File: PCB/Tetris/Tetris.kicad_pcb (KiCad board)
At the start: 2 copper layers, 101.6 x 53.3 mm, 27 parts, among them J1 Power, J2 PWM, J3 Analog, J4 PWM, J5 Analog, J6 Communication, J7 Digital, M1 RGBMatrix, M2 RGBMatrix, SW1 SW_Push, SW2 SW_Push, SW3 SW_Push, SW4 SW_Push, SW5 SW_Push, SW6 SW_Push, SW7 SW_Push

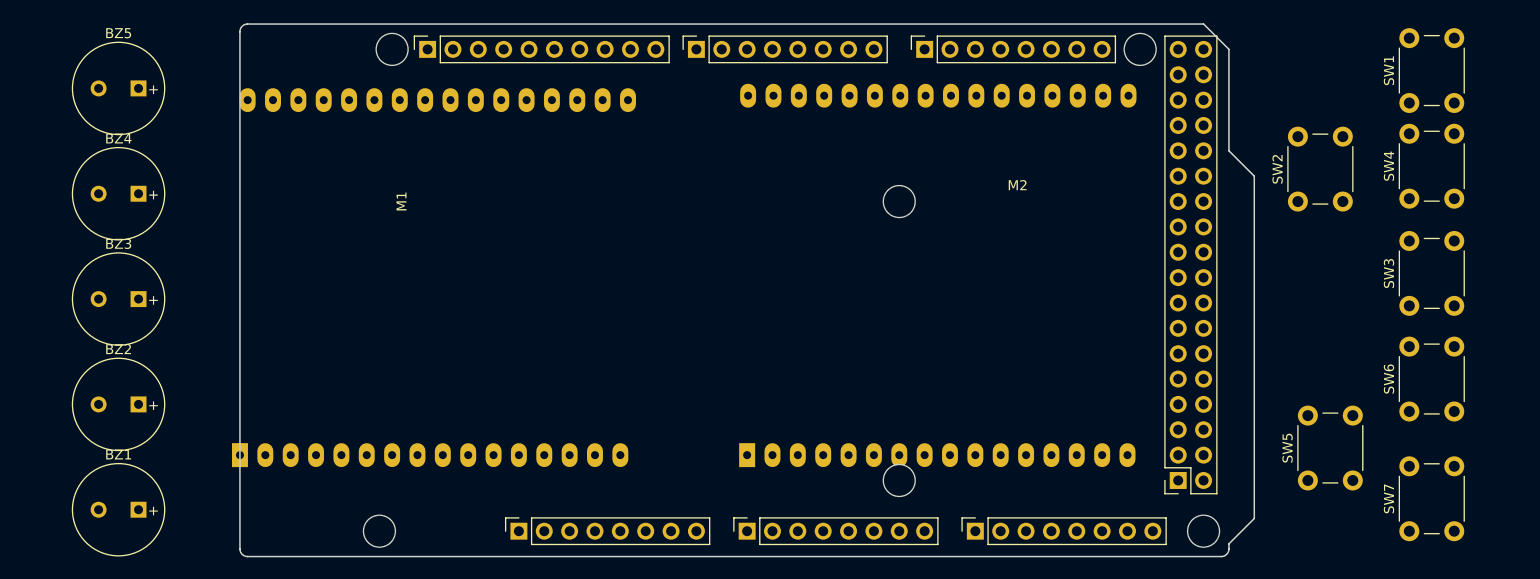
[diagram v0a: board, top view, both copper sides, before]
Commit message: sync
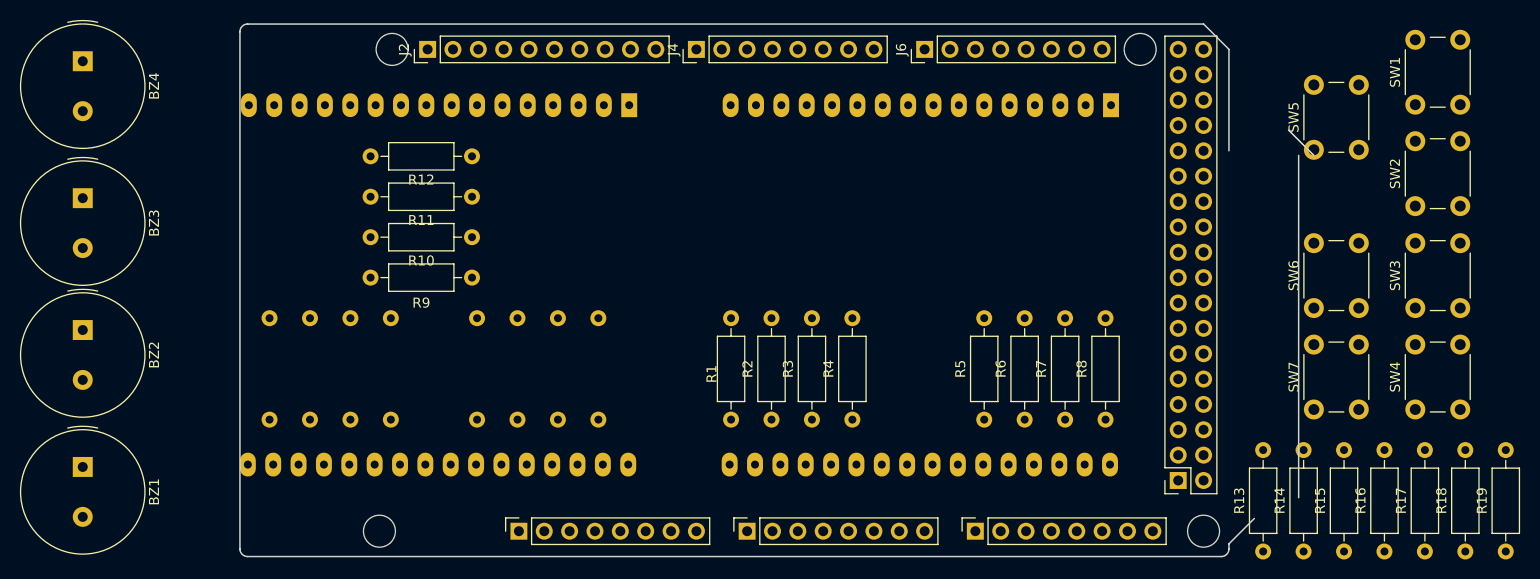
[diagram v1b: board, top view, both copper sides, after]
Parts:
- removed BZ5: Active Buzzer, Buzzer_Beeper:MagneticBuzzer_PUI_AT-0927-TT-6-R
- removed MH3, MH4: MountingHole_3.2mm, Arduino_MountingHole:MountingHole_3.2mm
- added R1: 110, Resistor_THT:R_Axial_DIN0207_L6.3mm_D2.5mm_P10.16mm_Horizontal, F.Cu at (149.2, 86.3)
- added R10: 220, Resistor_THT:R_Axial_DIN0207_L6.3mm_D2.5mm_P10.16mm_Horizontal, F.Cu at (123.2, 68.0)
- added R11: 220, Resistor_THT:R_Axial_DIN0207_L6.3mm_D2.5mm_P10.16mm_Horizontal, F.Cu at (123.2, 64.0)
- added R12: 220, Resistor_THT:R_Axial_DIN0207_L6.3mm_D2.5mm_P10.16mm_Horizontal, F.Cu at (123.2, 59.9)
- added R13: 10k, Resistor_THT:R_Axial_DIN0207_L6.3mm_D2.5mm_P10.16mm_Horizontal, F.Cu at (202.5, 99.5)
- added R14: 10k, Resistor_THT:R_Axial_DIN0207_L6.3mm_D2.5mm_P10.16mm_Horizontal, F.Cu at (206.5, 99.5)
- added R15: 10k, Resistor_THT:R_Axial_DIN0207_L6.3mm_D2.5mm_P10.16mm_Horizontal, F.Cu at (210.6, 99.5)
- added R16: 10k, Resistor_THT:R_Axial_DIN0207_L6.3mm_D2.5mm_P10.16mm_Horizontal, F.Cu at (214.6, 99.5)
- added R17: 10k, Resistor_THT:R_Axial_DIN0207_L6.3mm_D2.5mm_P10.16mm_Horizontal, F.Cu at (218.7, 99.5)
- added R18: 10k, Resistor_THT:R_Axial_DIN0207_L6.3mm_D2.5mm_P10.16mm_Horizontal, F.Cu at (222.7, 99.5)
- added R19: 10k, Resistor_THT:R_Axial_DIN0207_L6.3mm_D2.5mm_P10.16mm_Horizontal, F.Cu at (226.8, 99.5)
- added R2: 110, Resistor_THT:R_Axial_DIN0207_L6.3mm_D2.5mm_P10.16mm_Horizontal, F.Cu at (153.2, 86.3)
- added R20: 110, Resistor_THT:R_Axial_DIN0207_L6.3mm_D2.5mm_P10.16mm_Horizontal, B.Cu at (135.9, 86.3)
- added R21: 110, Resistor_THT:R_Axial_DIN0207_L6.3mm_D2.5mm_P10.16mm_Horizontal, B.Cu at (131.8, 86.3)
- added R22: 110, Resistor_THT:R_Axial_DIN0207_L6.3mm_D2.5mm_P10.16mm_Horizontal, B.Cu at (127.8, 86.3)
- added R23: 110, Resistor_THT:R_Axial_DIN0207_L6.3mm_D2.5mm_P10.16mm_Horizontal, B.Cu at (123.7, 86.3)
- added R24: 110, Resistor_THT:R_Axial_DIN0207_L6.3mm_D2.5mm_P10.16mm_Horizontal, B.Cu at (115.1, 86.3)
- added R25: 110, Resistor_THT:R_Axial_DIN0207_L6.3mm_D2.5mm_P10.16mm_Horizontal, B.Cu at (111.1, 86.3)
- added R26: 110, Resistor_THT:R_Axial_DIN0207_L6.3mm_D2.5mm_P10.16mm_Horizontal, B.Cu at (107.0, 86.3)
- added R27: 110, Resistor_THT:R_Axial_DIN0207_L6.3mm_D2.5mm_P10.16mm_Horizontal, B.Cu at (103.0, 86.3)
- added R3: 110, Resistor_THT:R_Axial_DIN0207_L6.3mm_D2.5mm_P10.16mm_Horizontal, F.Cu at (157.3, 86.3)
- added R4: 110, Resistor_THT:R_Axial_DIN0207_L6.3mm_D2.5mm_P10.16mm_Horizontal, F.Cu at (161.3, 86.3)
- added R5: 110, Resistor_THT:R_Axial_DIN0207_L6.3mm_D2.5mm_P10.16mm_Horizontal, F.Cu at (174.5, 86.3)
- added R6: 110, Resistor_THT:R_Axial_DIN0207_L6.3mm_D2.5mm_P10.16mm_Horizontal, F.Cu at (178.6, 86.3)
- added R7: 110, Resistor_THT:R_Axial_DIN0207_L6.3mm_D2.5mm_P10.16mm_Horizontal, F.Cu at (182.6, 86.3)
- added R8: 110, Resistor_THT:R_Axial_DIN0207_L6.3mm_D2.5mm_P10.16mm_Horizontal, F.Cu at (186.7, 86.3)
- added R9: 220, Resistor_THT:R_Axial_DIN0207_L6.3mm_D2.5mm_P10.16mm_Horizontal, F.Cu at (123.2, 72.1)
- BZ1, BZ2, BZ3, BZ4: footprint Buzzer_Beeper:MagneticBuzzer_PUI_AT-0927-TT-6-R -> Buzzer_Beeper:Buzzer_TDK_PS1240P02BT_D12.2mm_H6.5mm
- J2: footprint Connector_PinSocket_2.54mm:PinSocket_1x10_P2.54mm_Vertical -> Connector_PinHeader_2.54mm:PinHeader_1x10_P2.54mm_Vertical
- J4, J6: footprint Connector_PinSocket_2.54mm:PinSocket_1x08_P2.54mm_Vertical -> Connector_PinHeader_2.54mm:PinHeader_1x08_P2.54mm_Vertical
- moved M2 50.0 mm to (119.9, 72.8), turned to 180 degrees
- moved M1 49.6 mm to (168.1, 72.8), turned to 180 degrees
- moved SW5 33.1 mm to (207.6, 59.3)
- moved SW4 21.1 mm to (217.7, 85.3)
- moved SW7 15.5 mm to (207.6, 85.3)
- moved BZ4 14.4 mm to (84.3, 50.4), turned to -90 degrees
- moved SW6 14.1 mm to (207.6, 75.1)
- moved SW2 11.8 mm to (217.7, 64.9)
- moved BZ3 11.6 mm to (84.3, 64.1), turned to -90 degrees
- moved BZ2 9.31 mm to (84.3, 77.3), turned to -90 degrees
- moved BZ1 7.04 mm to (84.3, 91.0), turned to -90 degrees
- moved SW3 0.64 mm to (217.7, 75.1)
- moved SW1 0.62 mm to (217.7, 54.7)
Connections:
- M1 pad 10: /1 -> /10
- M1 pad 11: /1 -> /11
- M1 pad 12: /1 -> /12
- M1 pad 13: /1 -> /13
- M1 pad 14: /1 -> /14
- M1 pad 15: /1 -> /15
- M1 pad 16: /1 -> /16
- M1 pad 2: /1 -> /2
- M1 pad 21: /1 -> /21
- M1 pad 22: /1 -> /22
- M1 pad 23: /1 -> /23
- M1 pad 24: /1 -> /24
- M1 pad 25: /1 -> /25
- M1 pad 26: /1 -> /26
- M1 pad 27: /1 -> /27
- M1 pad 28: /1 -> /28
- M1 pad 3: /1 -> /3
- M1 pad 4: /1 -> /4
- M1 pad 5: /1 -> /5
- M1 pad 6: /1 -> /6
- M1 pad 7: /1 -> /7
- M1 pad 8: /1 -> /8
- M1 pad 9: /1 -> /9
- M2 pad 10: /1 -> /10
- M2 pad 11: /1 -> /11
- M2 pad 12: /1 -> /12
- M2 pad 13: /1 -> /13
- M2 pad 14: /1 -> /14
- M2 pad 15: /1 -> /15
- M2 pad 16: /1 -> /16
- M2 pad 2: /1 -> /2
- M2 pad 21: /1 -> /21
- M2 pad 22: /1 -> /22
- M2 pad 23: /1 -> /23
- M2 pad 24: /1 -> /24
- M2 pad 25: /1 -> /25
- M2 pad 26: /1 -> /26
- M2 pad 27: /1 -> /27
- M2 pad 28: /1 -> /28
- M2 pad 3: /1 -> /3
- M2 pad 4: /1 -> /4
- M2 pad 5: /1 -> /5
- M2 pad 6: /1 -> /6
- M2 pad 7: /1 -> /7
- M2 pad 8: /1 -> /8
- M2 pad 9: /1 -> /9
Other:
- board size 101.6 x 53.3 mm -> 107.6 x 53.3 mm
- board text removed: "ICSP"
